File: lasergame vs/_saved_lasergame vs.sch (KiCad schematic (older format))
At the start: 11 parts, among them J1 USB_B, J2 Screw_Terminal_01x02, SW1 SW_SPST, SW2 SW_Reed, U1 ATmega328-PU, Y1 Crystal

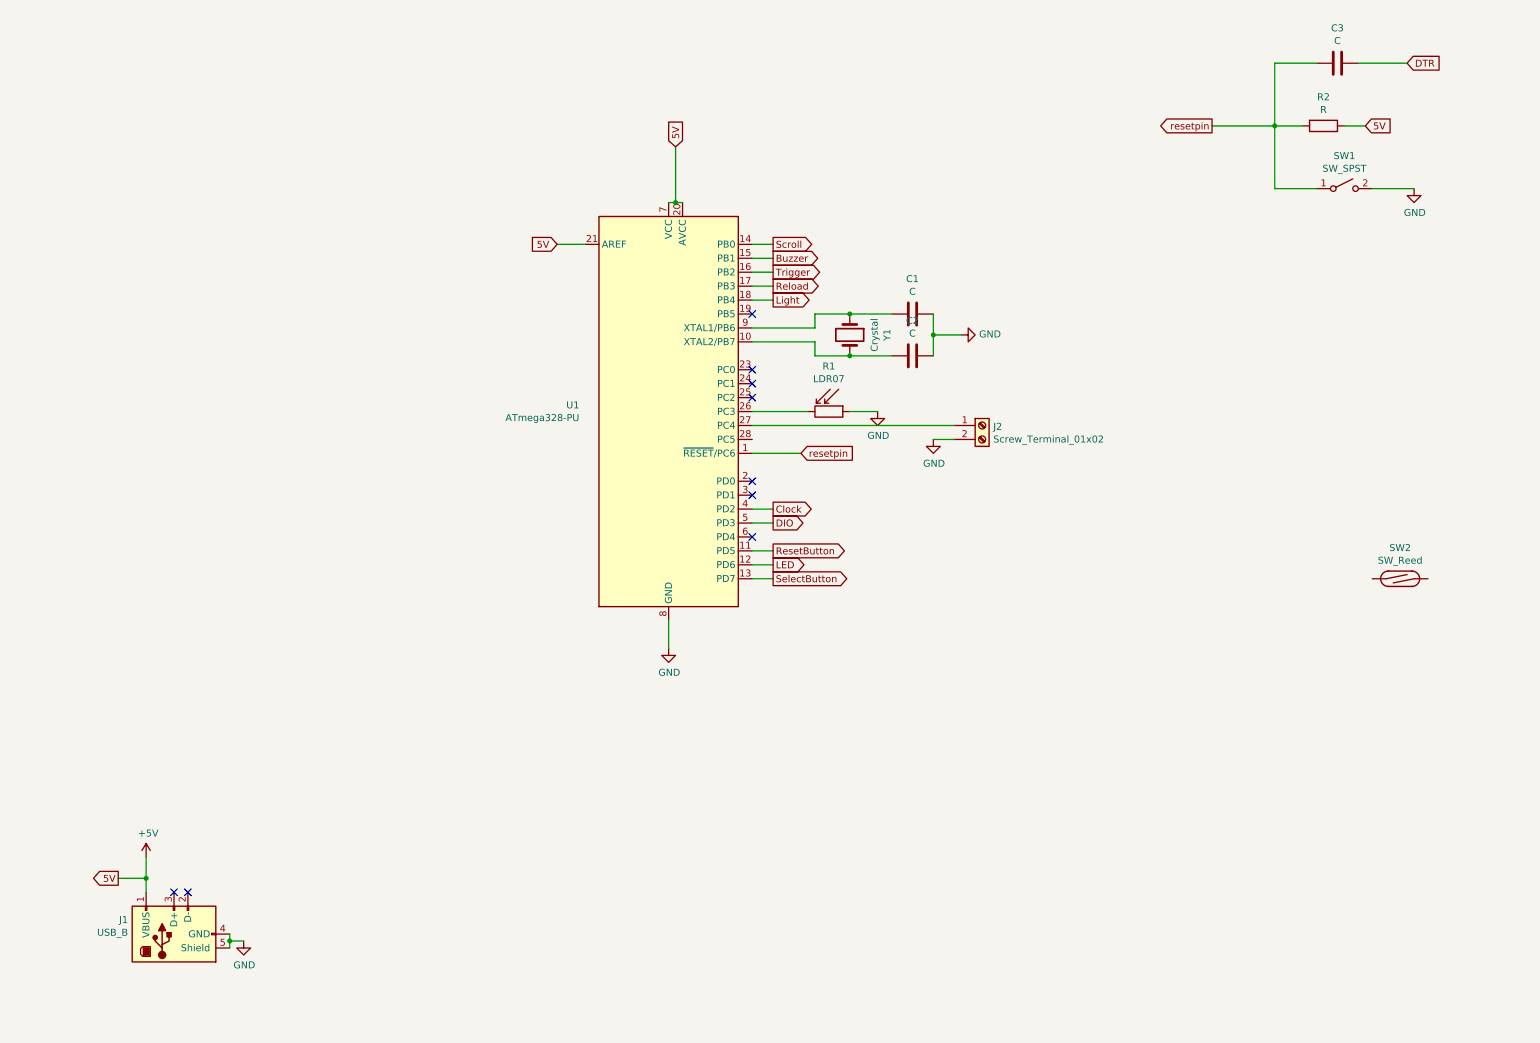
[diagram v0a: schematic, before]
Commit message: updated the schematics
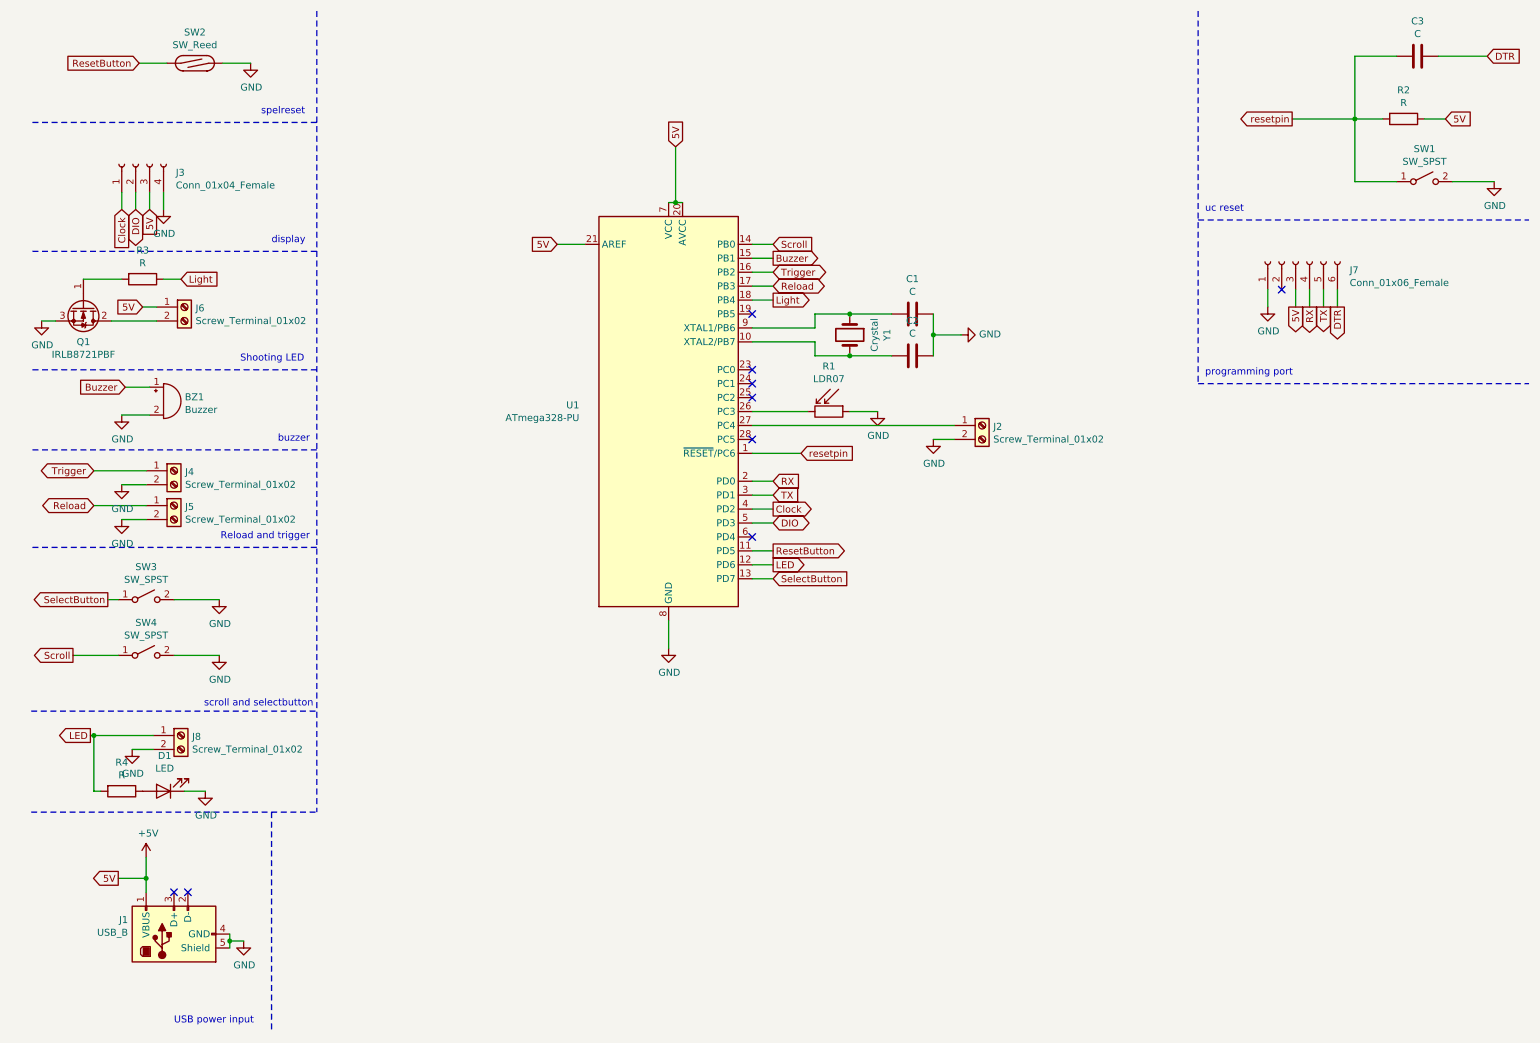
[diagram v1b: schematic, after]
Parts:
- added BZ1: Buzzer, symbol Device:Buzzer
- added D1: LED, symbol Device:LED
- added J3: Conn_01x04_Female, symbol Connector:Conn_01x04_Female
- added J4, J5, J6, J8: Screw_Terminal_01x02, symbol Connector:Screw_Terminal_01x02
- added J7: Conn_01x06_Female, symbol Connector:Conn_01x06_Female
- added Q1: IRLB8721PBF, Package_TO_SOT_THT:TO-220-3_Vertical, symbol Transistor_FET:IRLB8721PBF
- added R3, R4: R, symbol Device:R
- added SW3, SW4: SW_SPST, symbol Switch:SW_SPST
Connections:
- net +5V: now also J3.3 (Pin_3), J6.1 (Pin_1), J7.3 (Pin_3)
- net Buzzer: now also BZ1.1 (-)
- net Clock: now also J3.1 (Pin_1)
- net DIO: now also J3.2 (Pin_2)
- net DTR: now also J7.6 (Pin_6)
- net GND: now also SW2.2, BZ1.2 (+), D1.1 (K), J3.4 (Pin_4), J4.2 (Pin_2), J5.2 (Pin_2), J7.1 (Pin_1), J8.2 (Pin_2), Q1.3 (S), SW3.2 (B), SW4.2 (B)
- net LED: now also J8.1 (Pin_1), R4.2
- net Light: now also R3.1
- net Reload: now also J5.1 (Pin_1)
- net ResetButton: now also SW2.1
- net Scroll: now also SW4.1 (A)
- net SelectButton: now also SW3.1 (A)
- net Trigger: now also J4.1 (Pin_1)
- net RX: now reaches U1.2 (PD0)
- net RX: now also J7.4 (Pin_4)
- net TX: now reaches U1.3 (PD1)
- net TX: now also J7.5 (Pin_5)
- new net: Q1.1 (G), R3.2
- new net: J6.2 (Pin_2), Q1.2 (D)
- new net: D1.2 (A), R4.1
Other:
- note added: "Reload and trigger"
- note added: "Shooting LED"
- note added: "USB power input"
- note added: "buzzer"
- note added: "display"
- note added: "programming port"
- note added: "scroll and selectbutton"
- note added: "spelreset"
- note added: "uc reset"
- moved on the sheet: C3, R2, SW1, SW2
